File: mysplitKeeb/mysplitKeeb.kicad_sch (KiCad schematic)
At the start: 35 parts, among them Q1 Q_PNP_EBC, Q10 Q_PNP_EBC, Q11 Q_PNP_EBC, Q12 Q_PNP_EBC, Q13 Q_PNP_EBC, Q14 Q_PNP_EBC, Q15 Q_PNP_EBC, Q16 Q_PNP_EBC, Q17 Q_PNP_EBC, Q18 Q_PNP_EBC, Q19 Q_PNP_EBC, Q2 Q_PNP_EBC, Q20 Q_PNP_EBC, Q21 Q_PNP_EBC, Q22 Q_PNP_EBC, Q23 Q_PNP_EBC, Q24 Q_PNP_EBC, Q25 Q_PNP_EBC, Q26 Q_PNP_EBC, Q27 Q_PNP_EBC, Q28 Q_PNP_EBC, Q29 Q_PNP_EBC, Q3 Q_PNP_EBC, Q30 Q_PNP_EBC, Q4 Q_PNP_EBC, Q5 Q_PNP_EBC, Q6 Q_PNP_EBC, Q7 Q_PNP_EBC, Q8 Q_PNP_EBC, Q9 Q_PNP_EBC, U31 74HC4051, U32 74HC4051, U33 74HC4051, U34 74HC4051

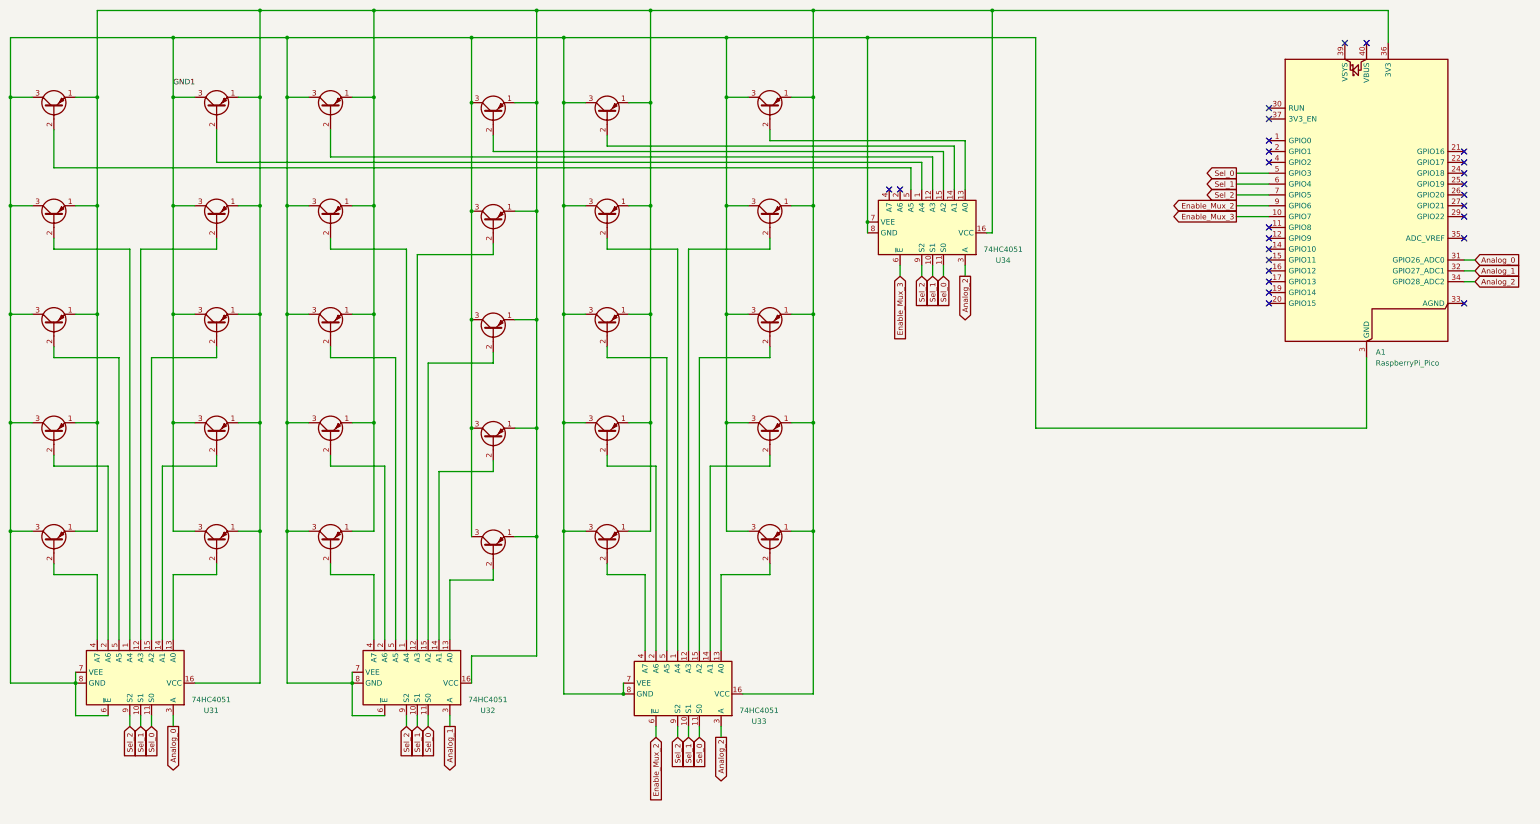
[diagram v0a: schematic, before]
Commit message: started new project
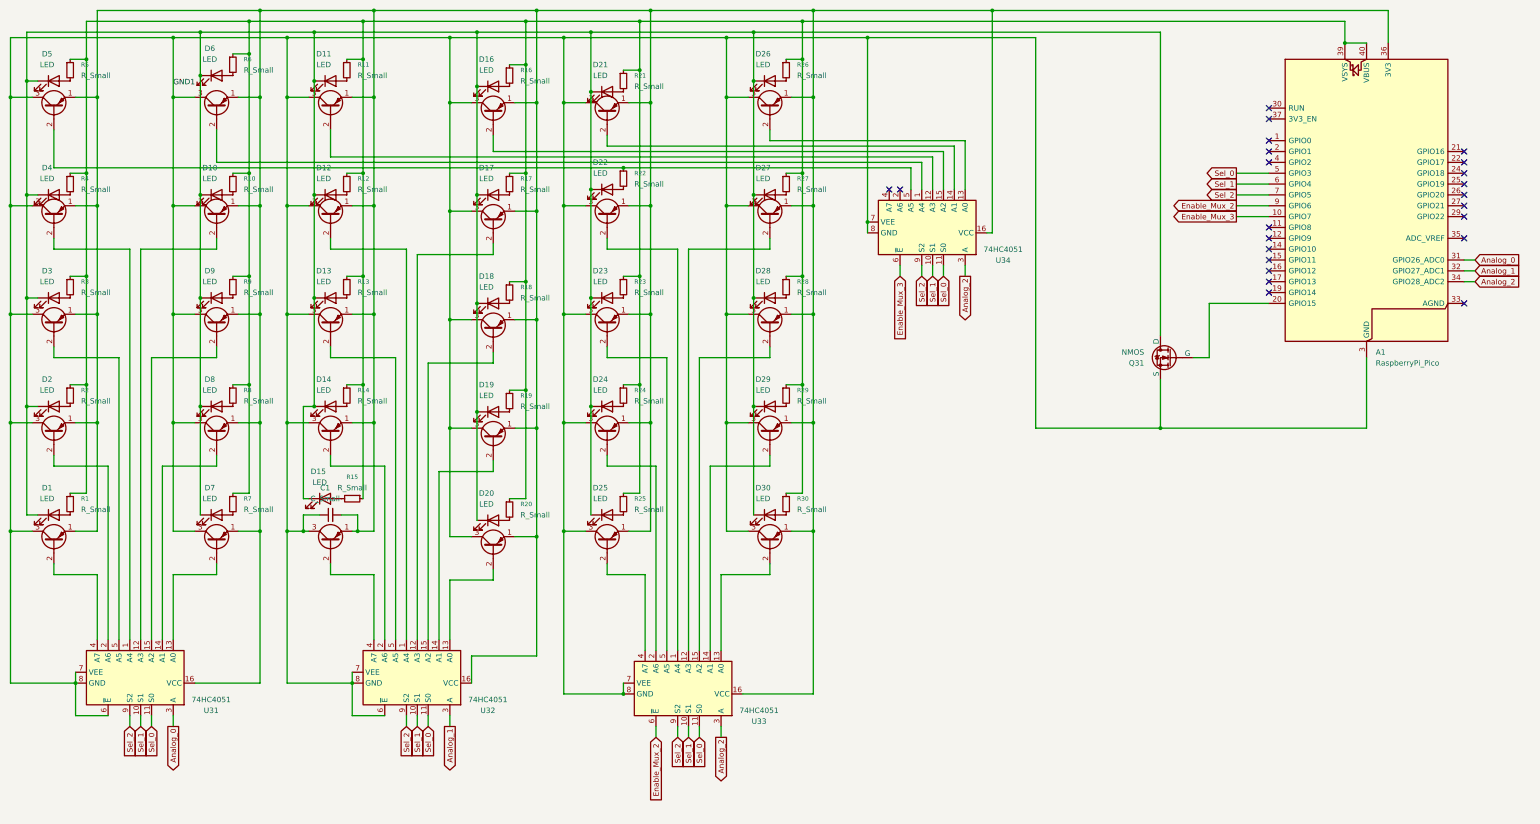
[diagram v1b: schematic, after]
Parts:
- added C1: C_Small, symbol Device:C_Small
- added D1, D10, D11, D12, D13, D14, D15, D16, D17, D18, D19, D2, D20, D21, D22, D23, D24, D25, D26, D27, D28, D29, D3, D30, D4, D5, D6, D7, D8, D9: LED, LED_SMD:LED_Everlight-SMD3528_3.5x2.8mm_67-21ST, symbol Device:LED
- added Q31: NMOS, Package_TO_SOT_SMD:SOT-23, symbol Simulation_SPICE:NMOS
- added R1, R10, R11, R12, R13, R14, R15, R16, R17, R18, R19, R2, R20, R21, R22, R23, R24, R25, R26, R27, R28, R29, R3, R30, R4, R5, R6, R7, R8, R9: R_Small, Resistor_SMD:R_1206_3216Metric_Pad1.30x1.75mm_HandSolder, symbol Device:R_Small
- U31, U32, U33, U34: footprint Package_DIP:DIP-16_W7.62mm -> Package_SO:SOIC-16_3.9x9.9mm_P1.27mm
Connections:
- net GND1: now also C1.1, Q31.3 (S)
- net at A1.36 (3V3), Q1.1 (E), Q10.1 (E)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: now also C1.2
- net at Q1.2 (B), U34.5 (A5): now also R22.1
- net at A1.20 (GPIO15): now also Q31.2 (G)
- net at A1.39 (VSYS): now also A1.40 (VBUS), R1.1, R10.1, R11.1, R12.1, R13.1, R14.1, R15.1, R16.1, R17.1, R18.1, R19.1, R2.1, R20.1, R21.1, R23.1, R24.1, R25.1, R26.1, R27.1, R28.1, R29.1, R3.1, R30.1, R4.1, R5.1, R6.1, R7.1, R8.1, R9.1
- new net: D5.2 (A), R5.2
- new net: D1.1 (K), D10.1 (K), D11.1 (K), D12.1 (K), D13.1 (K), D14.1 (K), D15.1 (K), D16.1 (K), D17.1 (K), D18.1 (K), D19.1 (K), D2.1 (K), D20.1 (K), D21.1 (K), D22.1 (K), D23.1 (K), D24.1 (K), D25.1 (K), D26.1 (K), D27.1 (K), D28.1 (K), D29.1 (K), D3.1 (K), D30.1 (K), D4.1 (K), D5.1 (K), D6.1 (K), D7.1 (K), D8.1 (K), D9.1 (K), Q31.1 (D)
- new net: D28.2 (A), R28.2
- new net: D23.2 (A), R23.2
- new net: D8.2 (A), R8.2
- new net: D19.2 (A), R19.2
- new net: D22.2 (A), R22.2
- new net: D18.2 (A), R18.2
- new net: D13.2 (A), R13.2
- new net: D15.2 (A), R15.2
- new net: D20.2 (A), R20.2
- new net: D6.2 (A), R6.2
- new net: D27.2 (A), R27.2
- new net: D3.2 (A), R3.2
- new net: D2.2 (A), R2.2
- new net: D1.2 (A), R1.2
- new net: D16.2 (A), R16.2
- new net: D7.2 (A), R7.2
- new net: D4.2 (A), R4.2
- new net: D30.2 (A), R30.2
- new net: D10.2 (A), R10.2
- new net: D9.2 (A), R9.2
- new net: D14.2 (A), R14.2
- new net: D21.2 (A), R21.2
- new net: D29.2 (A), R29.2
- new net: D24.2 (A), R24.2
- new net: D26.2 (A), R26.2
- new net: D11.2 (A), R11.2
- new net: D25.2 (A), R25.2
- new net: D12.2 (A), R12.2
- new net: D17.2 (A), R17.2
- no-connect marks 26 -> 23
